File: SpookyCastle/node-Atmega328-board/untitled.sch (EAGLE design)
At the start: 23 parts, among them IC2 MEGA48/88/168-AU

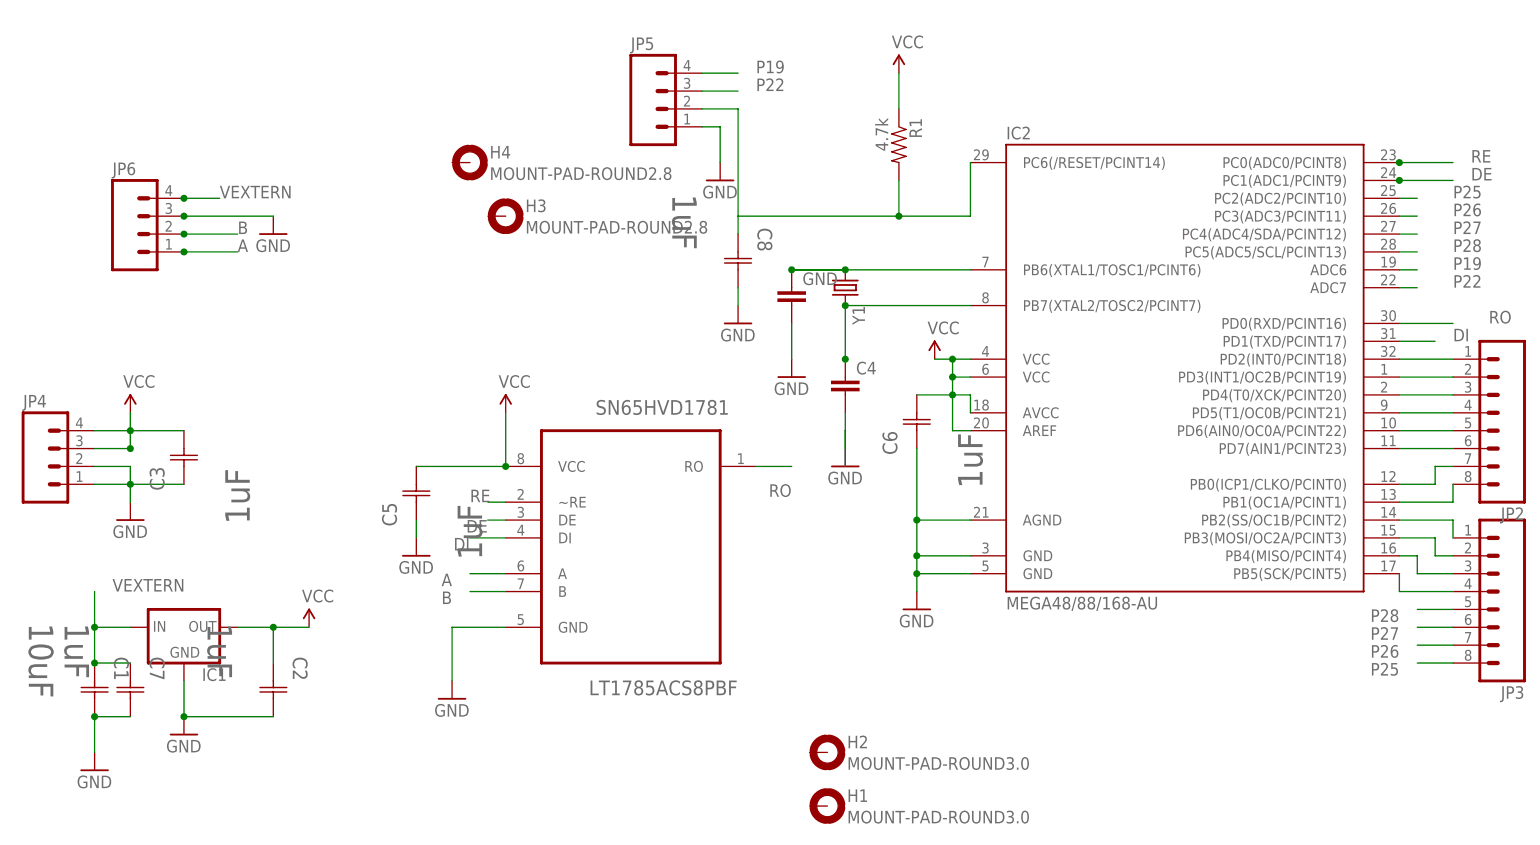
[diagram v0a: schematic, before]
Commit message: whole buncha changes
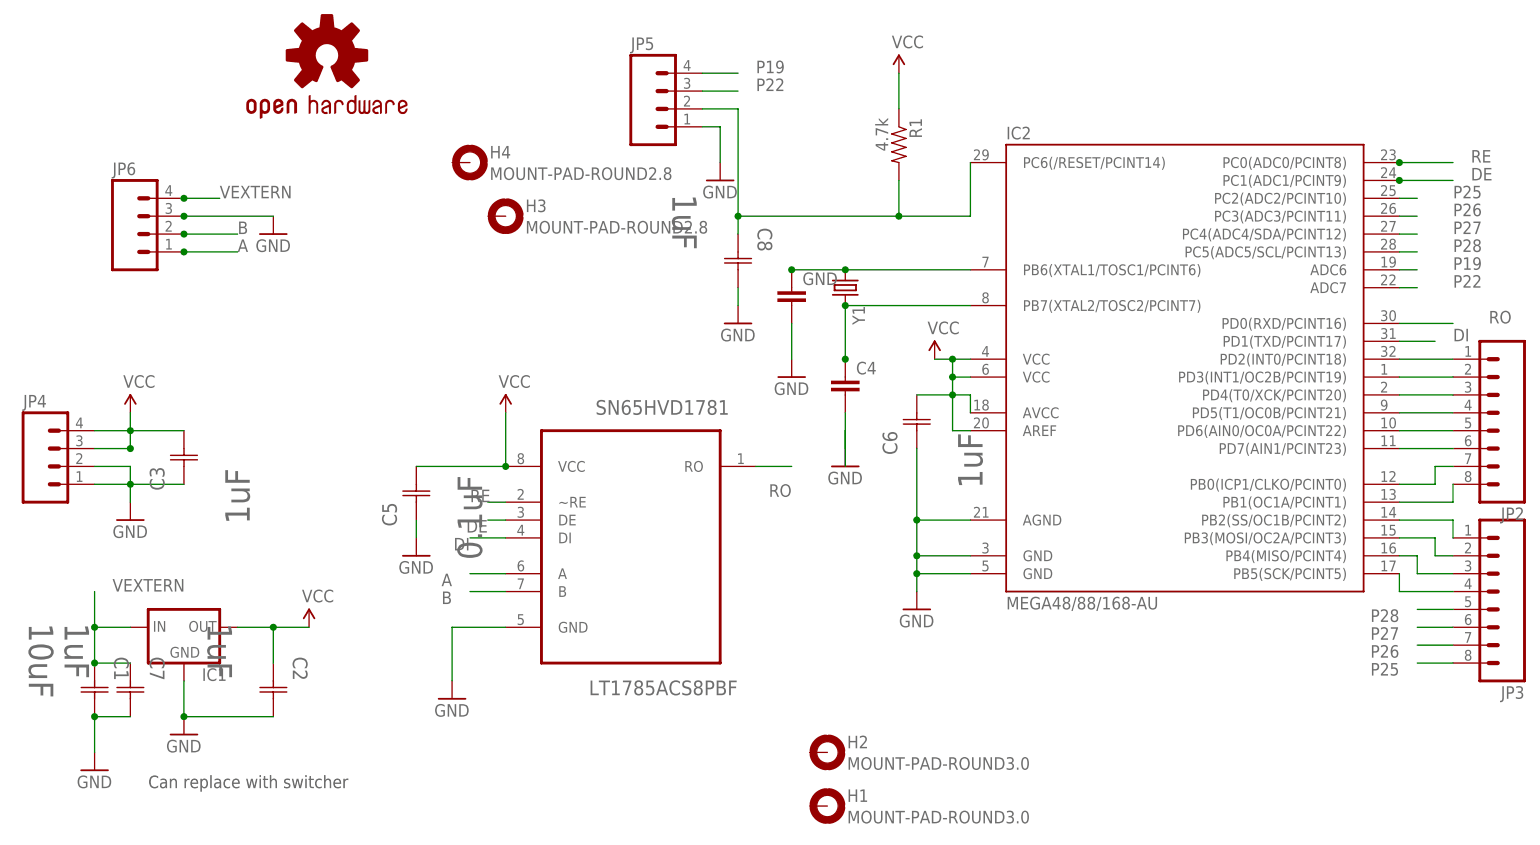
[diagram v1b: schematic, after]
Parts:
- added U$1: OSHW-LOGOM, SparkFun - Copy:OSHW-LOGOM
- C5: value 1uF -> 0.1uF
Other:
- note added: "Can replace with switcher"
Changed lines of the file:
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@@
 <part name="GND3" library="SparkFun - Copy" deviceset="GND" device=""/>
 <part name="GND4" library="SparkFun - Copy" deviceset="GND" device=""/>
-<part name="C5" library="Murata_By_element14_Batch_1" deviceset="GRM21BR71H105KA12L" device="" value="1uF">
+<part name="C5" library="Murata_By_element14_Batch_1" deviceset="GRM21BR71H105KA12L" device="" value="0.1uF">
 <attribute name="MPN" value="GRM21BR71H105KA12L "/>
 <attribute name="OC_FARNELL" value="1735541"/>
@@
 </part>
 <part name="JP6" library="SparkFun - Copy" deviceset="M04" device="SCREW"/>
+<part name="U$1" library="SparkFun - Copy" deviceset="OSHW-LOGO" device="M"/>
 </parts>
 <sheets>
 <sheet>
 <plain>
+<text x="-7.62" y="12.7" size="1.778" layer="97">Can replace with switcher</text>
 </plain>
 <instances>
@@
 <instance part="C8" gate="A" x="76.2" y="91.44" rot="R270"/>
 <instance part="JP6" gate="G$1" x="-7.62" y="91.44"/>
+<instance part="U$1" gate="G$1" x="17.78" y="116.84"/>
 </instances>
 <busses>
@@
 <segment>
 <pinref part="Y1" gate="G$1" pin="1"/>
-<wire x1="83.82" y1="86.36" x2="91.44" y2="86.36" width="0.1524" layer="91"/>
 <pinref part="GND" gate="G$1" pin="1"/>
 <junction x="83.82" y="86.36"/>
@@
 <pinref part="C8" gate="A" pin="C1"/>
 <wire x1="76.2" y1="91.44" x2="76.2" y2="93.98" width="0.1524" layer="91"/>
-</segment>
-</net>
+<junction x="76.2" y="93.98"/>
+</segment>
+</net>
